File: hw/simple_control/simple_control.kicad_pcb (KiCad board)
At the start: 4 copper layers, 99.1 x 99.1 mm, 87 parts, among them J101 Screw_Terminal_01x02, J102 Jack-DC, J103 Screw_Terminal_01x03, J104 Screw_Terminal_01x03, J1301 Micro_SD_Card, J1401 Conn_02x05_Odd_Even, J601 Conn_01x04, J602 Raspberry_Pi_0_2_3, J603 Conn_01x03, Q1001 BC817, Q201 AOSP21357, Q701 BC817, Q801 BC817, Q901 BC817, SW1201 SW_Push, SW601 SW_Push, U1101 CAT24C256, U301 SN74AHCT125D, U601 PicoW

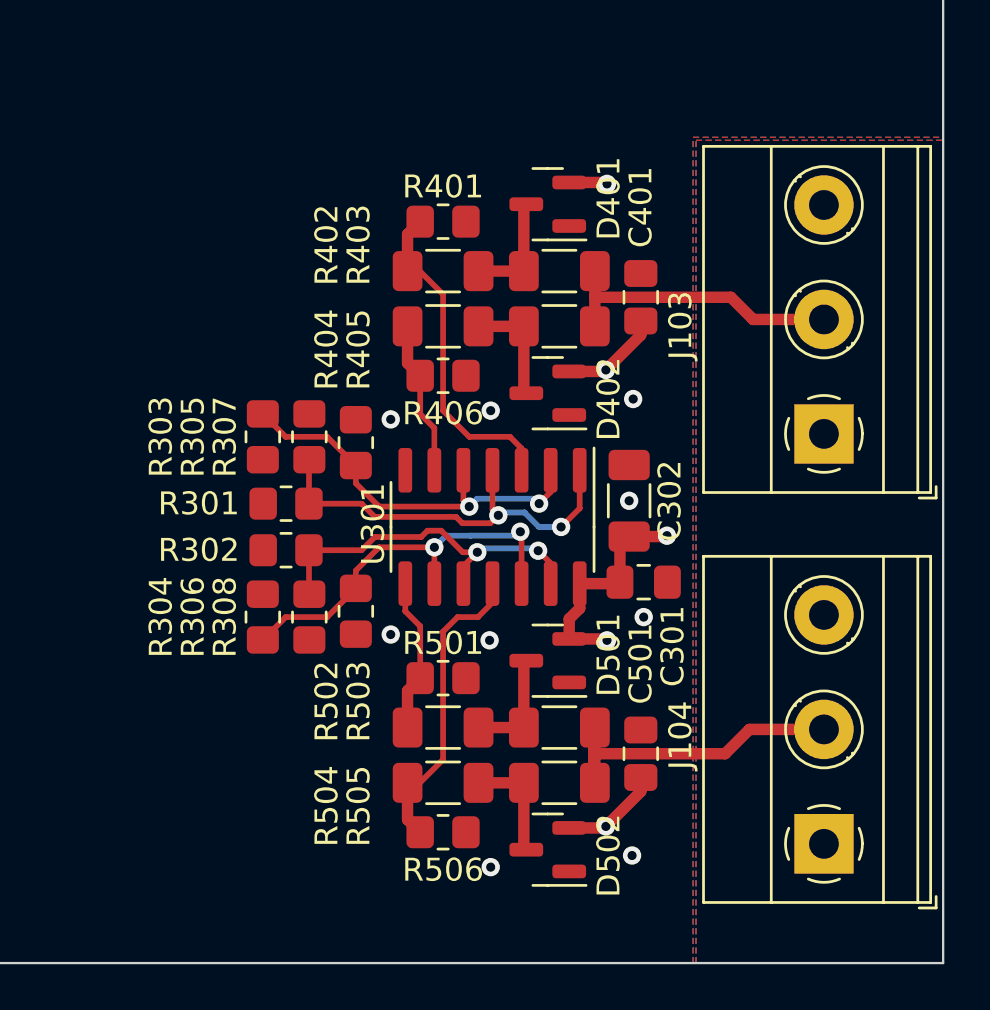
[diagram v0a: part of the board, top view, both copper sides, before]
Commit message: chore(hw): add led driver layout
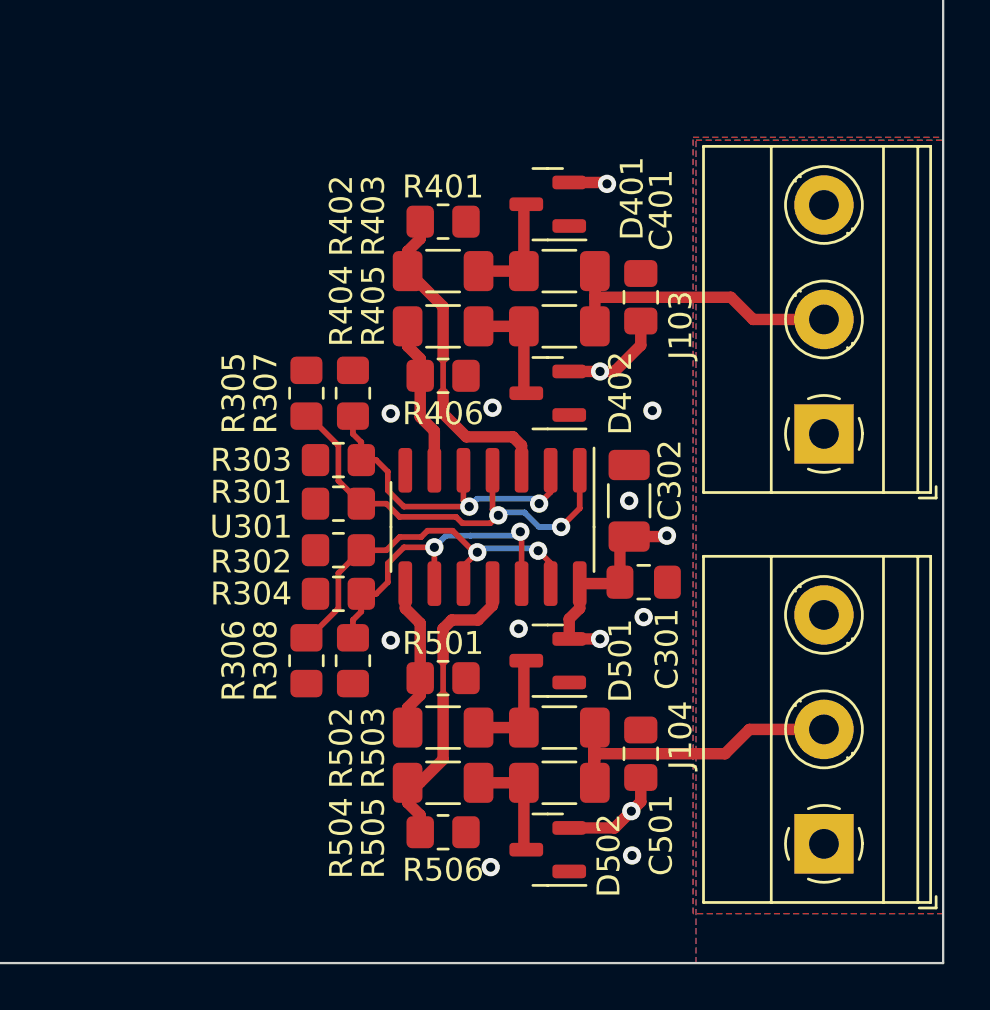
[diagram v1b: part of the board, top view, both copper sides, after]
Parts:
- moved R303 3.45 mm to (174.2, 117.7), turned to 0 degrees
- moved R304 3.45 mm to (174.2, 123.6), turned to 0 degrees
- moved R301 2.29 mm to (174.2, 119.6)
- moved R302 2.29 mm to (174.2, 121.7)
- moved R308 2.16 mm to (174.9, 126.5)
- moved R307 2.16 mm to (174.9, 114.8)
- moved R306 1.91 mm to (172.8, 126.5)
- moved R305 1.91 mm to (172.8, 114.8)
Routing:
- net +5V: track 31.7 -> 50.2 mm
- net Net-(U301-1A): track 17.8 -> 14.7 mm
- net Net-(U301-3A): track 17.5 -> 14.5 mm
- net Net-(U301-3~{OE}): track 16.1 -> 16.7 mm
- net Net-(U301-1~{OE}): track 18.6 -> 19.3 mm
